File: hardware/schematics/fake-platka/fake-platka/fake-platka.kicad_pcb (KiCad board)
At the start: 2 copper layers, 196.8 x 74.9 mm, 88 parts, among them J1 XT60PW-F, J10 B2B-EH-A, J11 B2B-EH-A, J12 B2B-EH-A, J13 B2B-EH-A, J14 XT60PW-F, J15 XT60PW-F, J16 B2B-EH-A, J17 B2B-EH-A, J18 B2B-EH-A, J19 B2B-EH-A, J2 XT60PW-F, J20 B2B-EH-A, J21 XT60PW-F, J22 XT60PW-F, J23 B2B-EH-A, J24 B2B-EH-A, J25 B2B-EH-A, J26 B2B-EH-A, J27 B2B-EH-A, J28 XT60PW-F, J29 XT60PW-F, J3 B2B-EH-A, J30 B2B-EH-A, J4 B2B-EH-A, J5 B2B-EH-A, J6 B2B-EH-A, J7 XT60PW-F, J8 XT60PW-F, J9 B2B-EH-A, U1 XL4005, U10 TB67H450AFNG_EL, U11 TB67H450AFNG_EL, U12 TB67H450AFNG_EL, U2 XL4005, U3 SC0915-pico-w-board, U4 SC0915-pico-w-board, U5 TB67H450AFNG_EL, U6 TB67H450AFNG_EL, U7 TB67H450AFNG_EL, U8 TB67H450AFNG_EL, U9 TB67H450AFNG_EL

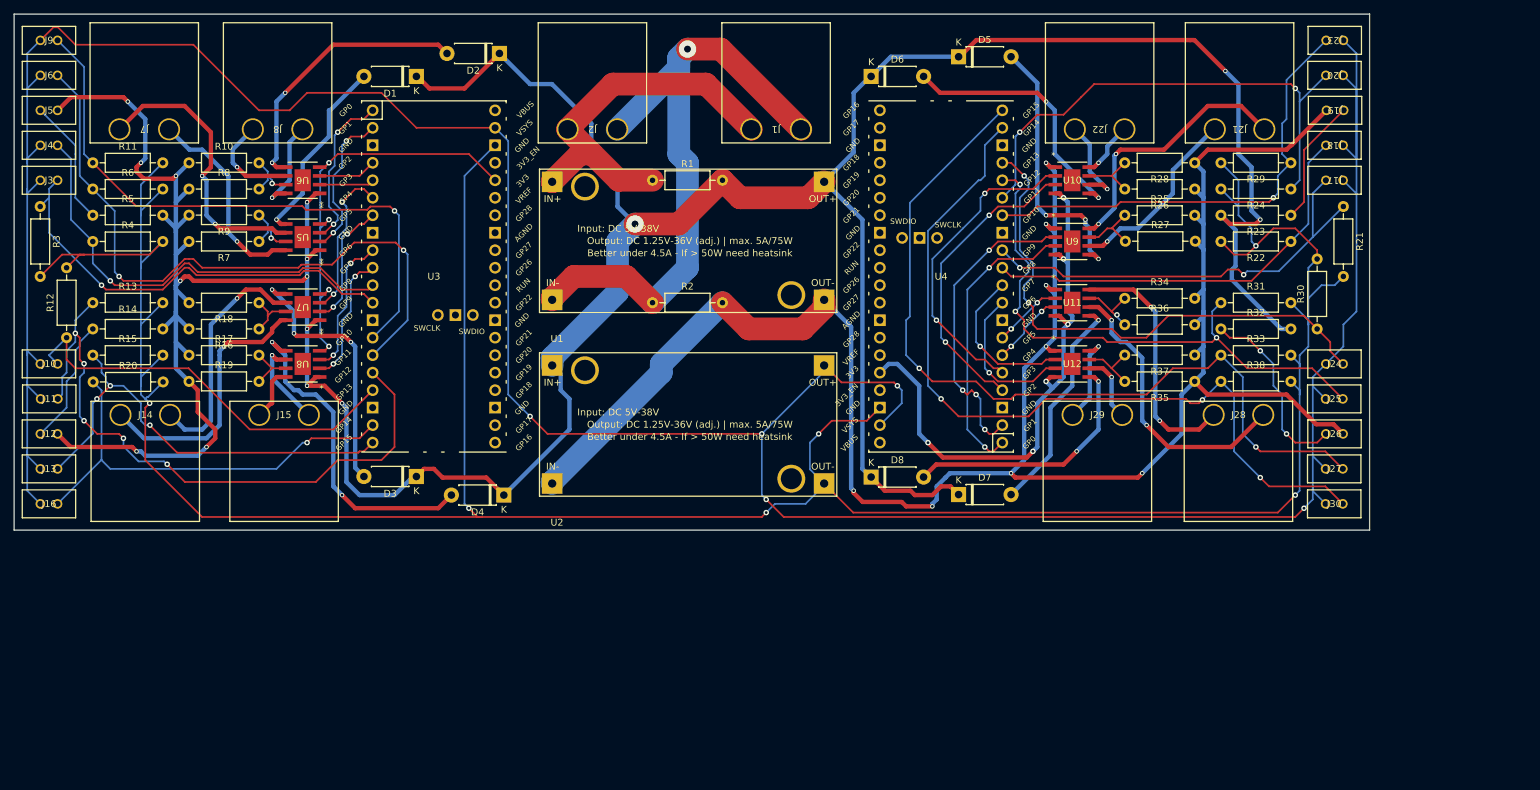
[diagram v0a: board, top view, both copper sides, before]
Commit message: finalizing the documentation
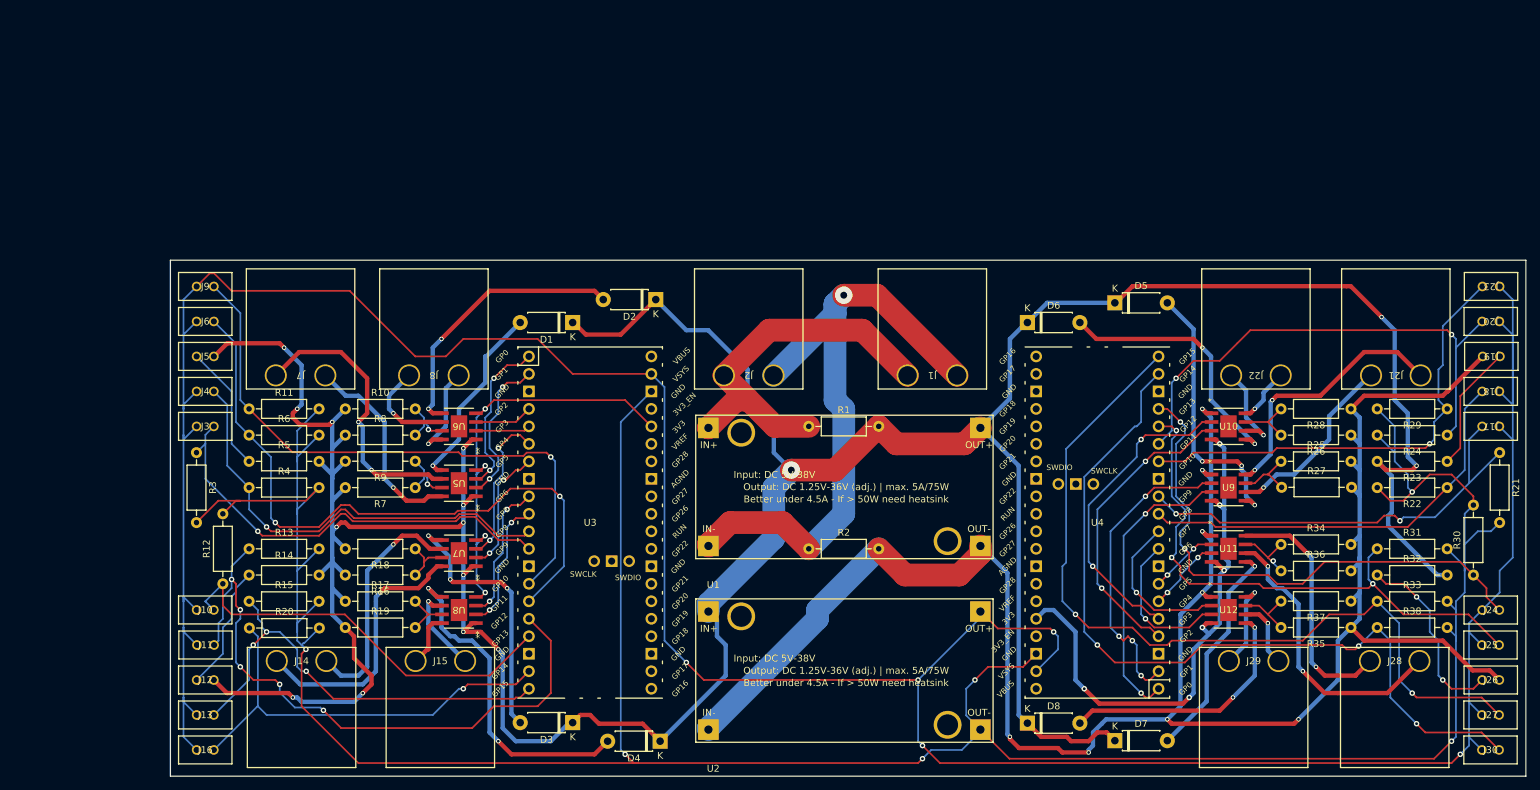
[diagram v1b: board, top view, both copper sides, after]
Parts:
- moved J23 42.3 mm to (247.5, 72.6)
- moved R21 42.3 mm to (247.5, 96.7)
- moved R23 42.3 mm to (239.9, 98.0)
- moved R25 42.3 mm to (215.7, 98.0)
- moved R28 42.3 mm to (225.9, 90.3)
- moved R29 42.3 mm to (239.9, 90.3)
- moved R30 42.3 mm to (243.7, 114.5)
- moved R32 42.3 mm to (229.7, 114.5)
- moved R33 42.3 mm to (229.7, 118.3)
- moved R35 42.3 mm to (225.9, 122.1)
- moved R36 42.3 mm to (215.7, 113.9)
- moved R37 42.3 mm to (225.9, 118.3)
- moved R38 42.3 mm to (229.7, 122.1)
- moved U10 42.3 mm to (208.1, 92.9)
- moved U12 42.3 mm to (208.1, 119.6)
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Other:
- board size 196.8 x 74.9 mm -> 196.9 x 74.9 mm
